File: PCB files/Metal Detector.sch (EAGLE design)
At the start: 14 parts, among them IC1 NE5534AD, Q1 IRF740, Q2 BC556, T1 BC547, X1 A1944-50

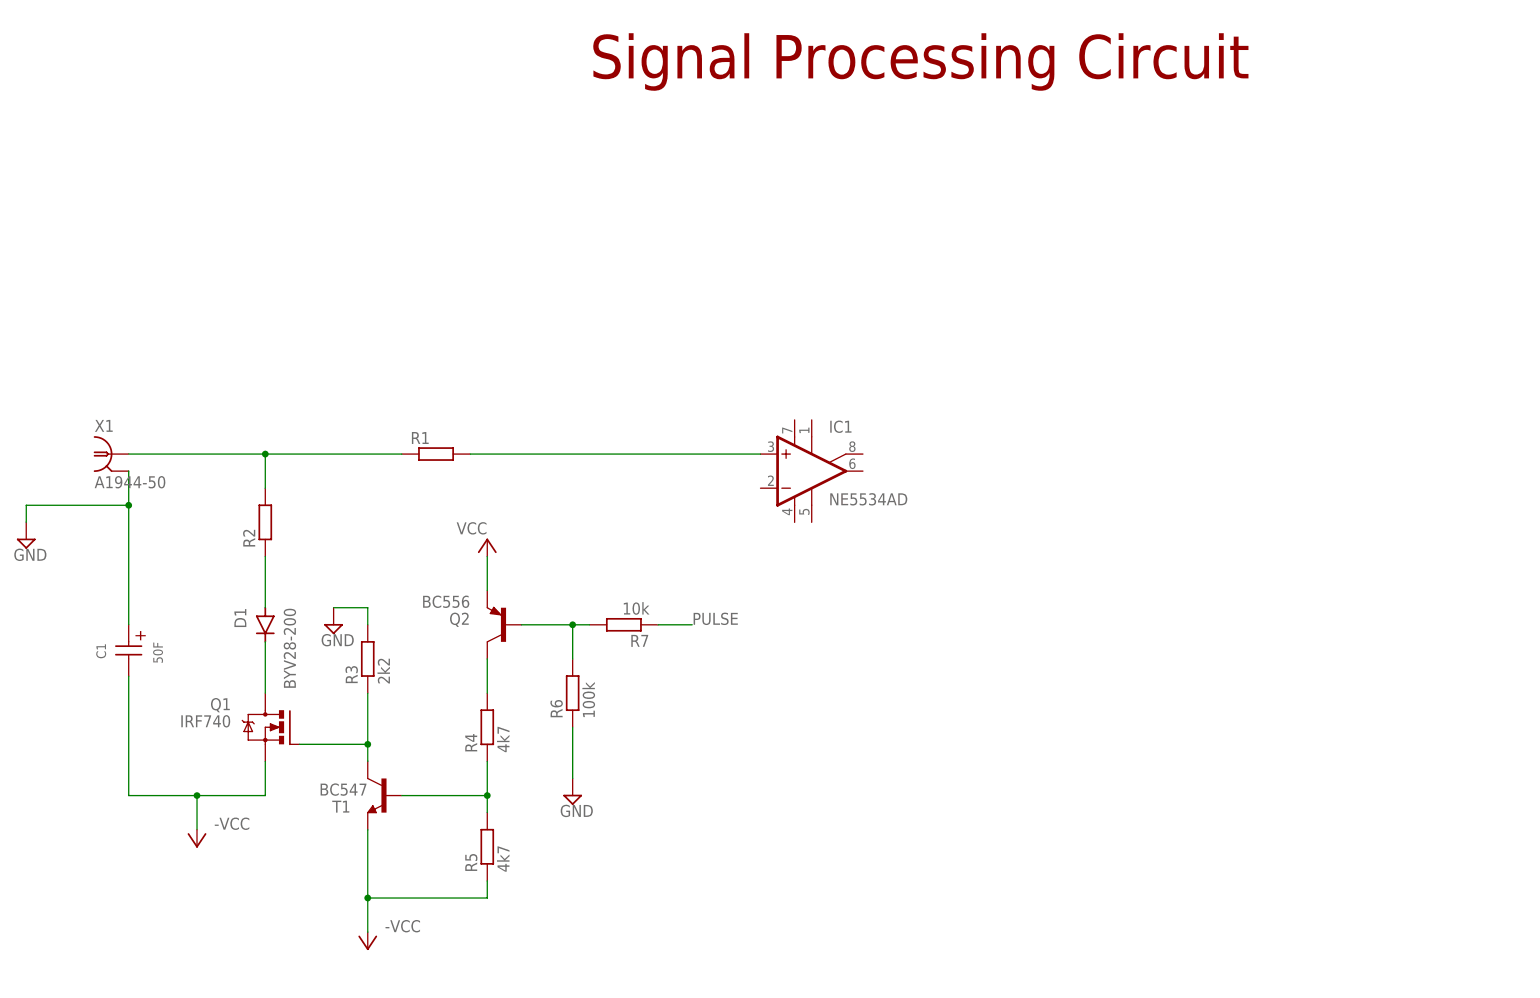
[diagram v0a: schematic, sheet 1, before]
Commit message: Add files via upload
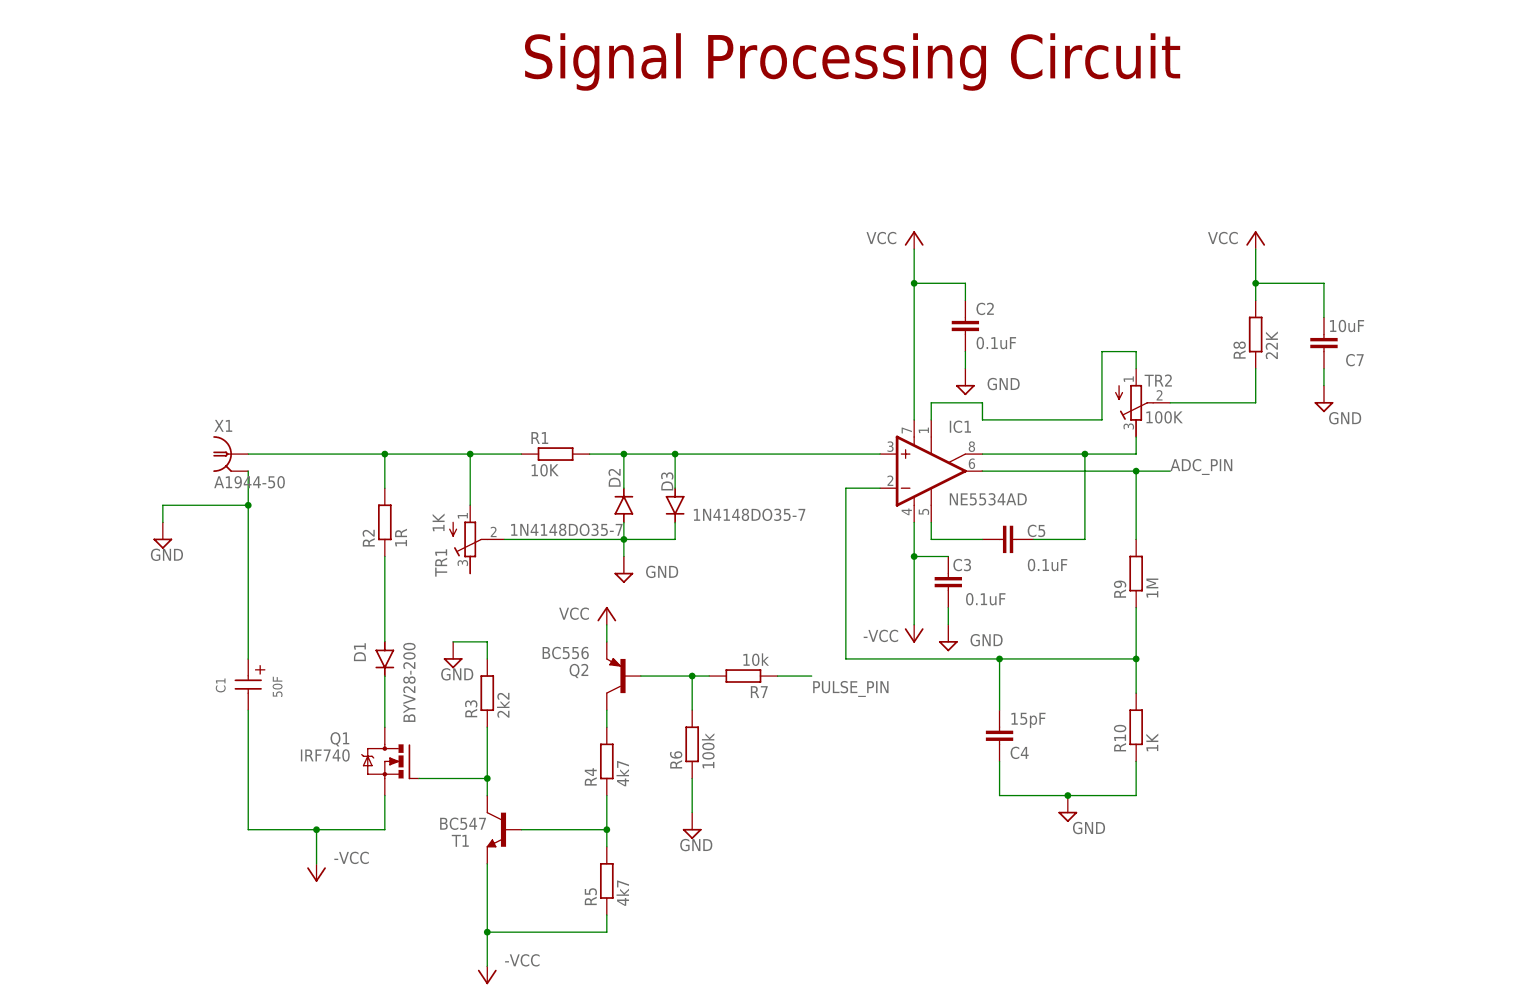
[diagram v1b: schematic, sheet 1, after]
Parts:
- added C2, C3, C5: 0.1uF, SparkFun-Capacitors:0.1UF-0402-6.3V-10%-X7R
- added C4: 15pF, SparkFun-Capacitors:0.1UF-0402-6.3V-10%-X7R
- added C7: 10uF, SparkFun-Capacitors:10UF-0402T-6.3V-20%
- added D2, D3: 1N4148DO35-7, diode:1N4148DO35-7
- added R10: 1K, rcl:R-EU_0207/10
- added R8: 22K, rcl:R-EU_0207/10
- added R9: 1M, rcl:R-EU_0207/10
- added TR1: 1K, rcl:R-TRIMM3296X
- added TR2: 100K, rcl:R-TRIMM3296X
- R1: value (none) -> 10K
- R2: value (none) -> 1R
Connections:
- net PULSE renamed PULSE_PIN
- new net ADC_PIN: IC1.OUT, R9.2
- new net N$10: R8.1, TR2.S
- new net N$11: C5.2, IC1.ON/CMP, TR2.E
- new net N$12: C4.2, IC1.-IN, R10.2, R9.1
- new net N$13: C5.1, IC1.CMP
- new net N$9: IC1.ON, TR2.A
- net GND: now also C2.2, C3.2, C4.1, C7.1, D2.A, D3.C, R10.1, TR1.S
- net N$1: now also TR1.A
- net N$2: now also D2.C, D3.A
- net VCC: now also C2.1, C3.1, C7.2, IC1.V+, IC1.V-, R8.2
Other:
- moved on the sheet: C1, D1, IC1, Q1, Q2, R1, R2, R3, R4, R5, R6, R7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
